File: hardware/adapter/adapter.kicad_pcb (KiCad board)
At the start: 2 copper layers, 37.3 x 45.9 mm, 29 parts, among them J1 Conn_01x01_Pin, J10 Conn_01x01_Pin, J11 Conn_01x01_Pin, J12 Conn_01x01_Pin, J13 Conn_01x01_Pin, J14 Conn_01x01_Pin, J15 Conn_01x01_Pin, J16 Conn_01x01_Pin, J17 Conn_01x01_Pin, J18 Conn_01x01_Pin, J19 Conn_01x01_Pin, J2 Conn_01x01_Pin, J20 Conn_01x01_Pin, J21 Conn_01x01_Pin, J22 Conn_01x01_Pin, J23 Conn_01x01_Pin, J24 Conn_01x01_Pin, J25 Conn_01x01_Pin, J26 Conn_01x01_Pin, J27 Conn_01x01_Pin, J28 Conn_01x01_Pin, J3 Conn_01x01_Pin, J4 Conn_01x01_Pin, J5 Conn_01x01_Pin, J6 Conn_01x01_Pin, J7 Conn_01x01_Pin, J8 Conn_01x01_Pin, J9 Conn_01x01_Pin, U2 MAX2121ETI+

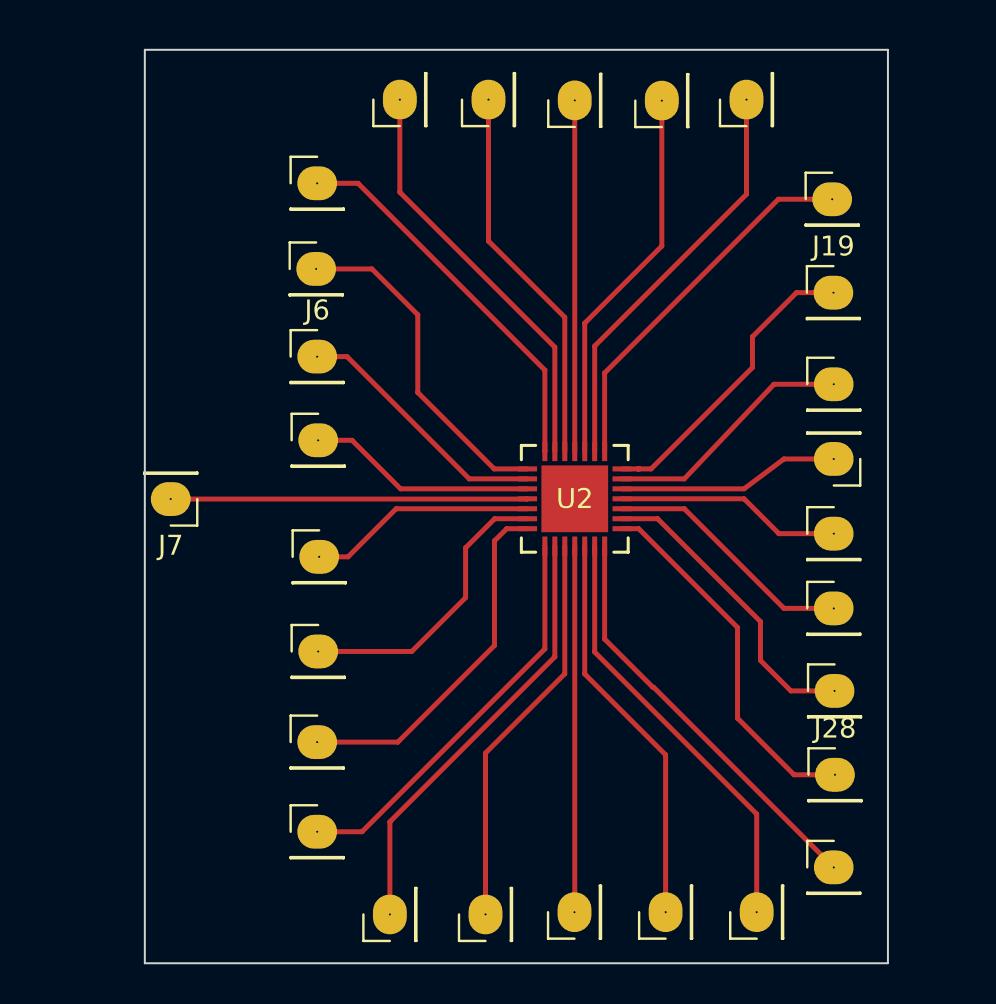
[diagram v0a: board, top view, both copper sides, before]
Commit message: new space offset
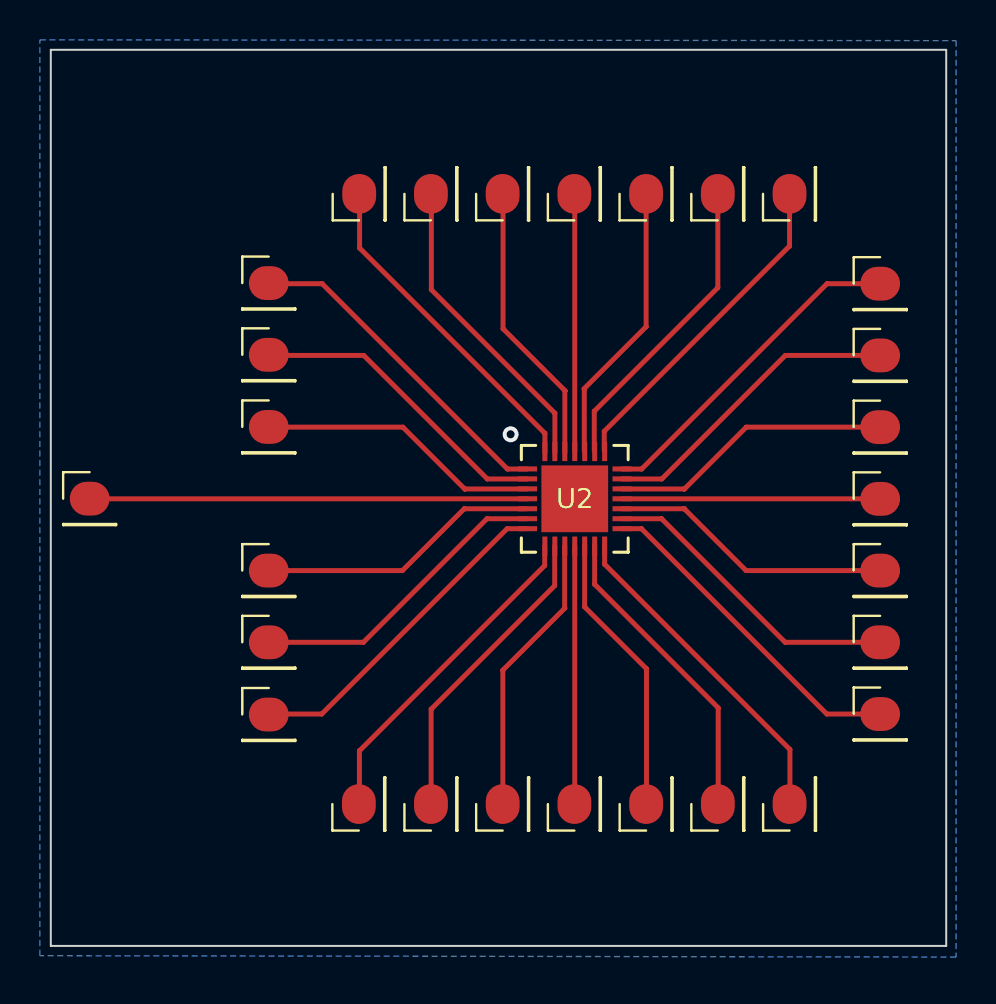
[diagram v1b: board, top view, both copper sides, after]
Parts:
- moved J12 5.91 mm to (144.0, 111.2)
- moved J15 5.77 mm to (158.4, 111.2)
- moved J13 5.61 mm to (147.6, 111.2)
- moved J14 5.51 mm to (154.8, 111.2)
- moved J17 5.43 mm to (151.2, 111.2)
- moved J25 4.98 mm to (144.0, 80.5)
- moved J21 4.94 mm to (158.4, 80.5)
- moved J24 4.78 mm to (147.6, 80.5)
- moved J22 4.75 mm to (154.8, 80.5)
- moved J23 4.69 mm to (151.2, 80.5)
- moved J7 4.07 mm to (126.8, 95.8), turned to 0 degrees
- moved J16 3.87 mm to (162.0, 111.2), turned to 90 degrees
- moved J28 3.80 mm to (166.5, 106.6)
- moved J27 3.35 mm to (166.5, 103.0)
- moved J5 3.00 mm to (166.5, 99.4)
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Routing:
- net Net-(J12-Pin_1): track 21.9 -> 15.5 mm
- net Net-(J15-Pin_1): track 21.7 -> 15.5 mm
- net Net-(J13-Pin_1): track 20.1 -> 14.2 mm
- net Net-(J14-Pin_1): track 20.1 -> 14.2 mm
- net Net-(J17-Pin_1): track 18.4 -> 13.0 mm
- net Net-(J25-Pin_1): track 20.9 -> 15.5 mm
- net Net-(J21-Pin_1): track 20.8 -> 15.5 mm
- net Net-(J24-Pin_1): track 19.3 -> 14.2 mm
- net Net-(J22-Pin_1): track 19.2 -> 14.2 mm
- net Net-(J23-Pin_1): track 17.6 -> 12.9 mm
- net Net-(J16-Pin_1): track 20.9 -> 16.8 mm
- net Net-(J7-Pin_1): track 17.9 -> 22.0 mm
- net Net-(J11-Pin_1): track 20.4 -> 16.8 mm
- net Net-(J3-Pin_1): track 11.1 -> 14.2 mm
- net Net-(J2-Pin_1): track 12.7 -> 15.5 mm
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- added copper zone on B.Cu, net (none)
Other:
- board size 37.3 x 45.9 mm -> 44.9 x 45 mm
